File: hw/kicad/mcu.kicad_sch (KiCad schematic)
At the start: 44 parts, among them J20 USB_A, J21 USB_B_Micro, U10 LPC55S16JBD100, U11 PRTR5V0U2X.215, U12 PRTR5V0U2X.215, Y1 32khz, Y2 16Mhz

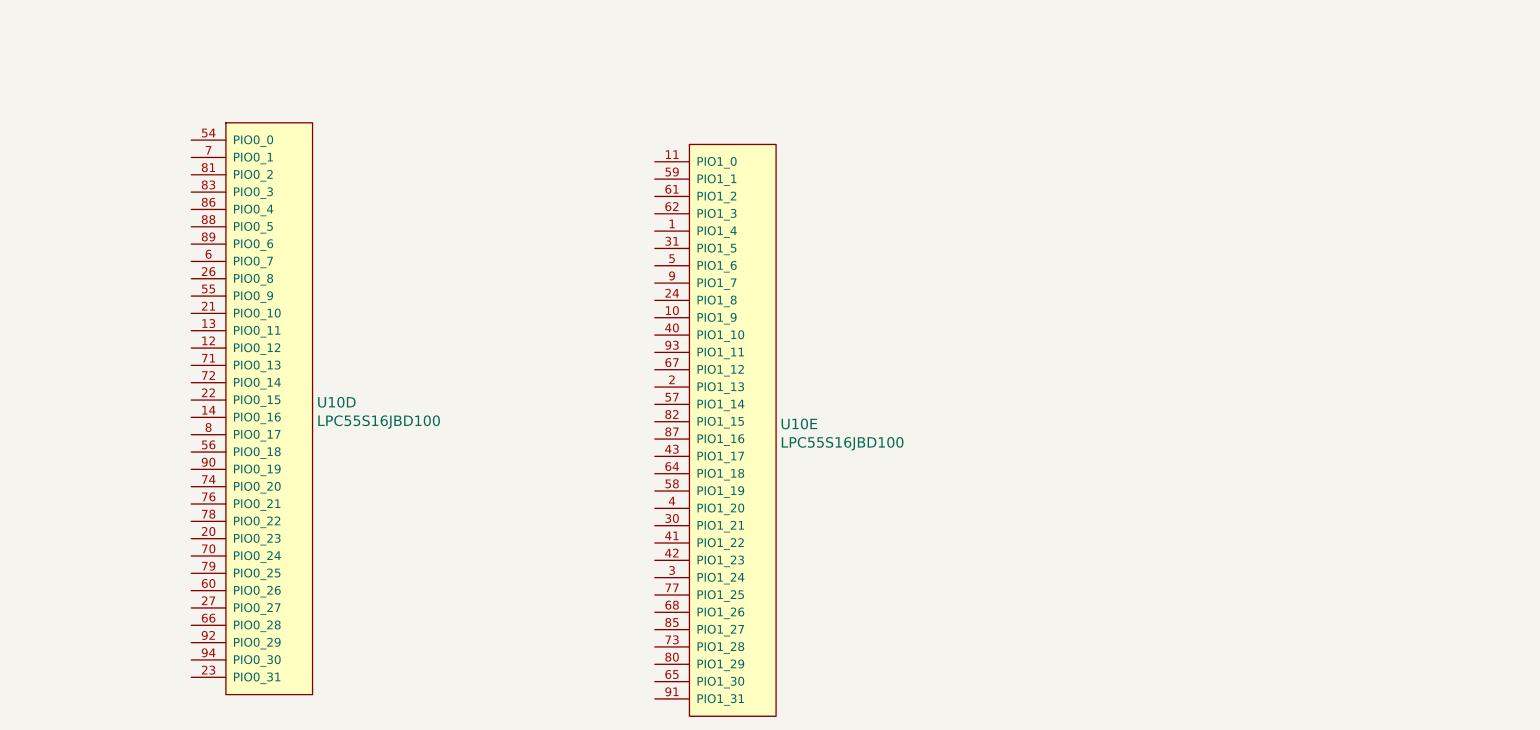
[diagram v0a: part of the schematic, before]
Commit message: hw schematics
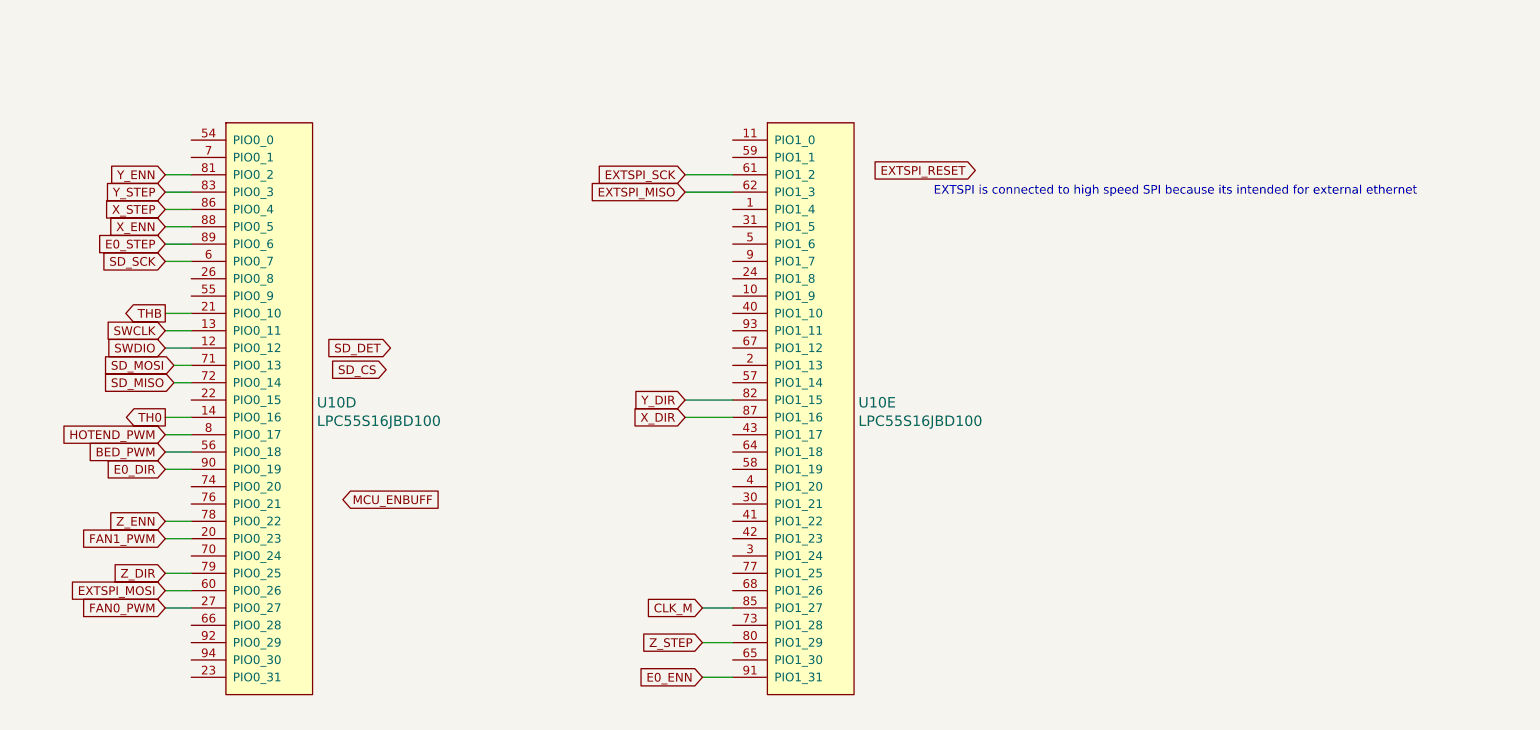
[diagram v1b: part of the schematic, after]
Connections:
- net EXTSPI_SCK: now reaches U10.61 (PIO1_2)
- net EXTSPI_MISO: now reaches U10.62 (PIO1_3)
- net Z_STEP: now reaches U10.80 (PIO1_29)
- net Y_DIR: now reaches U10.82 (PIO1_15)
- net CLK_M: now reaches U10.85 (PIO1_27)
- net X_DIR: now reaches U10.87 (PIO1_16)
- net E0_ENN: now reaches U10.91 (PIO1_31)
- net SWDIO: now reaches U10.12 (PIO0_12)
- net SWCLK: now reaches U10.13 (PIO0_11)
- net TH0: now reaches U10.14 (PIO0_16)
- net FAN1_PWM: now reaches U10.20 (PIO0_23)
- net THB: now reaches U10.21 (PIO0_10)
- net FAN0_PWM: now reaches U10.27 (PIO0_27)
- net BED_PWM: now reaches U10.56 (PIO0_18)
- net SD_SCK: now reaches U10.6 (PIO0_7)
- net EXTSPI_MOSI: now reaches U10.60 (PIO0_26)
- net SD_MOSI: now reaches U10.71 (PIO0_13)
- net SD_MISO: now reaches U10.72 (PIO0_14)
- net Z_ENN: now reaches U10.78 (PIO0_22)
- net Z_DIR: now reaches U10.79 (PIO0_25)
- net HOTEND_PWM: now reaches U10.8 (PIO0_17)
- net Y_ENN: now reaches U10.81 (PIO0_2)
- net Y_STEP: now reaches U10.83 (PIO0_3)
- net X_STEP: now reaches U10.86 (PIO0_4)
- net X_ENN: now reaches U10.88 (PIO0_5)
- net E0_STEP: now reaches U10.89 (PIO0_6)
- net E0_DIR: now reaches U10.90 (PIO0_19)
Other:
- note added: "EXTSPI is connected to high speed SPI because its intended for external ethernet"
- moved on the sheet: U10E
